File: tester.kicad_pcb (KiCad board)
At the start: 2 copper layers, 55.9 x 40.6 mm, 13 parts

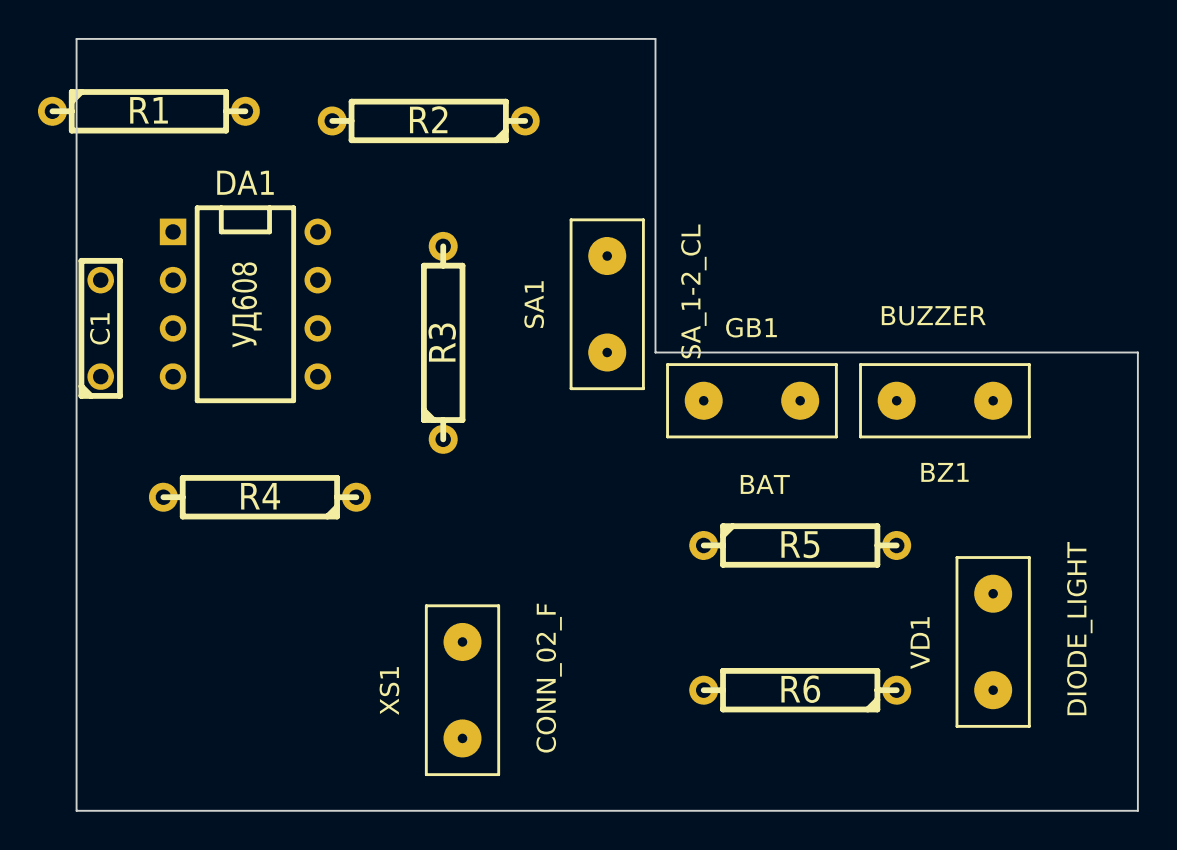
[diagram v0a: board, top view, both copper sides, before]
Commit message: next step
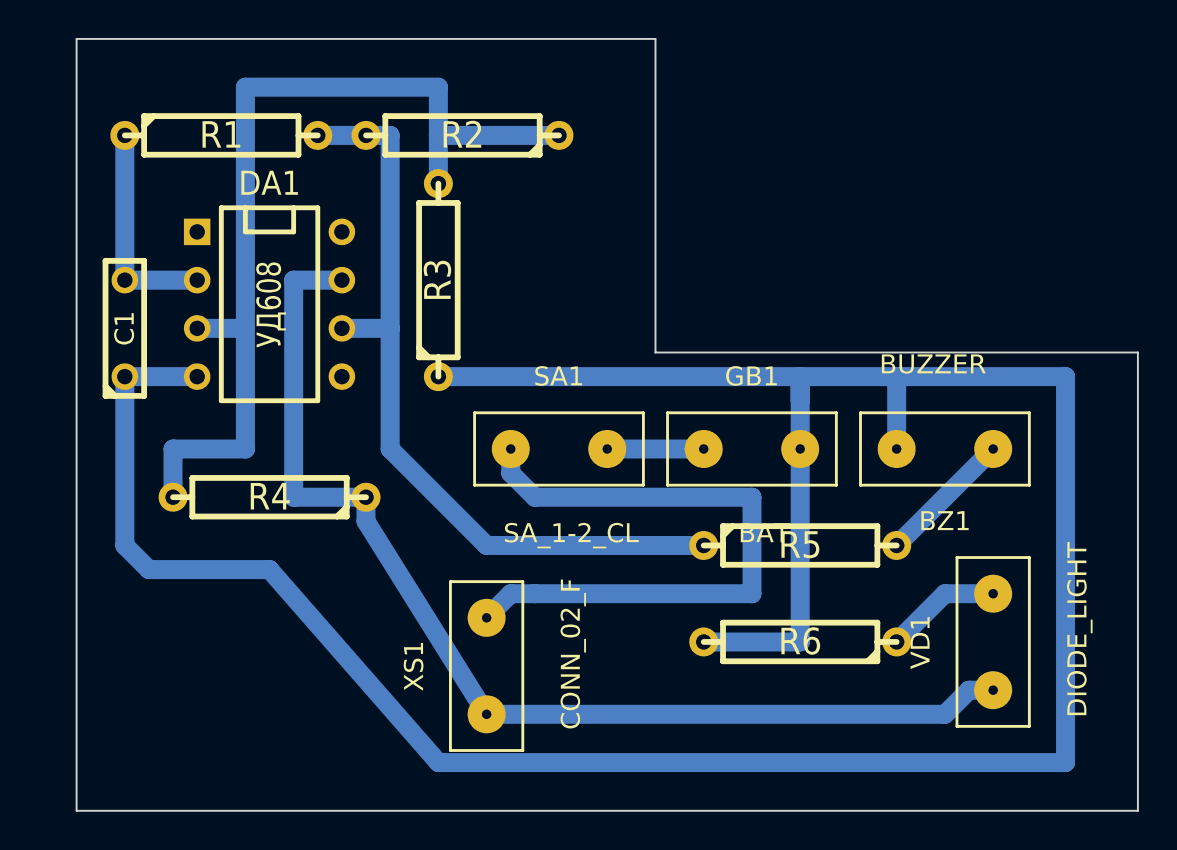
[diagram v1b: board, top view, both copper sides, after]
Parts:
- moved SA1 8.03 mm to (45.7, 55.9), turned to 0 degrees
- moved R1 4.02 mm to (27.9, 39.4)
- moved R3 3.31 mm to (39.4, 47.0)
- moved BZ1 2.54 mm to (66.0, 55.9)
- moved GB1 2.54 mm to (55.9, 55.9)
- moved R6 2.54 mm to (58.4, 66.0)
- moved R2 1.93 mm to (40.6, 39.4)
- moved XS1 1.80 mm to (41.9, 67.3)
- moved C1 1.27 mm to (22.9, 49.5)
- moved DA1 1.27 mm to (30.5, 48.3)
- moved R4 0.51 mm to (30.5, 58.4)
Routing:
- net GND: track 0.00 -> 144.8 mm
- net N-000008: track 0.00 -> 58.2 mm
- net N-000004: track 0.00 -> 49.5 mm
- net N-000009: track 0.00 -> 41.5 mm
- net N-000001: track 0.00 -> 34.1 mm
- net N-000007: track 0.00 -> 11.4 mm
- net N-000005: track 0.00 -> 7.18 mm
- net N-000002: track 0.00 -> 6.13 mm
- net N-000003: track 0.00 -> 5.08 mm
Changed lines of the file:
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@@
-(kicad_pcb (version 3) (host pcbnew "(2013-jul-07)-stable")
+(kicad_pcb (version 3) (host pcbnew "(2013-07-07 BZR 4022)-stable")
   (general
     (links 20)
-    (no_connects 20)
-    (area 20.269999 34.137599 78.486 78.934)
+    (no_connects 0)
+    (area 18.034 34.239999 76.250001 74.980001)
     (thickness 1.6)
     (drawings 6)
-    (tracks 0)
+    (tracks 53)
     (zones 0)
     (modules 13)
@@
   )
   (setup
-    (last_trace_width 0.254)
+    (last_trace_width 1)
+    (user_trace_width 0.5)
+    (user_trace_width 1)
     (trace_clearance 0.254)
     (zone_clearance 0.508)
@@
     (pad_to_mask_clearance 0)
     (aux_axis_origin 0 0)
-    (visible_elements 7FFFF591)
+    (visible_elements 7FFF2511)
     (pcbplotparams
       (layerselection 3178497)
@@
   )
   (module R4   placed (layer F.Cu)
-    (at 24.13 38.1)
+    (at 27.94 39.37)
     (descr "Resitance 4 pas")
     (tags R)
@@
   )
   (module R4   placed (layer F.Cu)
-    (at 39.624 50.292 90)
+    (at 39.37 46.99 90)
     (descr "Resitance 4 pas")
     (tags R)
@@
   )
   (module R4   placed (layer F.Cu)
-    (at 29.972 58.42 180)
+    (at 30.48 58.42 180)
     (descr "Resitance 4 pas")
     (tags R)
@@
   )
   (module R4   placed (layer F.Cu)
-    (at 38.862 38.608 180)
+    (at 40.64 39.37 180)
     (descr "Resitance 4 pas")
     (tags R)
@@
   )
   (module DIP-8__300   placed (layer F.Cu)
-    (at 29.21 48.26 270)
+    (at 30.48 48.26 270)
     (descr "8 pins DIL package, round pads")
     (tags DIL)
@@
   )
   (module C2   placed (layer F.Cu)
-    (at 21.59 49.53 90)
+    (at 22.86 49.53 90)
     (descr "Condensateur = 2 pas")
     (tags C)
@@
   )
   (module R4 (layer F.Cu)
-    (at 58.42 68.58 180)
+    (at 58.42 66.04 180)
     (descr "Resitance 4 pas")
     (tags R)
@@
   )
   (module Con2 (layer F.Cu)
-    (at 55.88 53.34)
+    (at 55.88 55.88)
     (fp_text reference GB1 (at 0 -3.81) (layer F.SilkS)
       (effects (font (size 1 1) (thickness 0.15)))
@@
   )
   (module Con2 (layer F.Cu)
-    (at 40.64 68.58 90)
+    (at 41.91 67.31 90)
     (fp_text reference XS1 (at 0 -3.81 90) (layer F.SilkS)
       (effects (font (size 1 1) (thickness 0.15)))
@@
   )
   (module Con2 (layer F.Cu)
-    (at 48.26 48.26 90)
-    (fp_text reference SA1 (at 0 -3.81 90) (layer F.SilkS)
-      (effects (font (size 1 1) (thickness 0.15)))
-    )
-    (fp_text value SA_1-2_CL (at 0.635 4.445 90) (layer F.SilkS)
+    (at 45.72 55.88)
+    (fp_text reference SA1 (at 0 -3.81) (layer F.SilkS)
+      (effects (font (size 1 1) (thickness 0.15)))
+    )
+    (fp_text value SA_1-2_CL (at 0.635 4.445) (layer F.SilkS)
+      (effects (font (size 1 1) (thickness 0.15)))
+    )
+    (fp_line (start -4.445 -1.905) (end 4.445 -1.905) (layer F.SilkS) (width 0.15))
+    (fp_line (start 4.445 -1.905) (end 4.445 1.905) (layer F.SilkS) (width 0.15))
+    (fp_line (start 4.445 1.905) (end -4.445 1.905) (layer F.SilkS) (width 0.15))
+    (fp_line (start -4.445 1.905) (end -4.445 -1.905) (layer F.SilkS) (width 0.15))
+    (pad 1 thru_hole circle (at -2.54 0) (size 2 2) (drill 0.5)
+      (layers *.Cu *.Mask F.SilkS)
+      (net 2 N-000001)
+    )
+    (pad 2 thru_hole circle (at 2.54 0) (size 2 2) (drill 0.5)
+      (layers *.Cu *.Mask F.SilkS)
+      (net 4 N-000003)
+    )
+  )
+  (module Con2 (layer F.Cu)
+    (at 68.58 66.04 90)
+    (fp_text reference VD1 (at 0 -3.81 90) (layer F.SilkS)
+      (effects (font (size 1 1) (thickness 0.15)))
+    )
+    (fp_text value DIODE_LIGHT (at 0.635 4.445 90) (layer F.SilkS)
       (effects (font (size 1 1) (thickness 0.15)))
     )
@@
     (pad 1 thru_hole circle (at -2.54 0 90) (size 2 2) (drill 0.5)
       (layers *.Cu *.Mask F.SilkS)
-      (net 2 N-000001)
+      (net 8 N-000008)
     )
     (pad 2 thru_hole circle (at 2.54 0 90) (size 2 2) (drill 0.5)
       (layers *.Cu *.Mask F.SilkS)
-      (net 4 N-000003)
+      (net 3 N-000002)
     )
   )
   (module Con2 (layer F.Cu)
-    (at 68.58 66.04 90)
-    (fp_text reference VD1 (at 0 -3.81 90) (layer F.SilkS)
-      (effects (font (size 1 1) (thickness 0.15)))
-    )
-    (fp_text value DIODE_LIGHT (at 0.635 4.445 90) (layer F.SilkS)
-      (effects (font (size 1 1) (thickness 0.15)))
-    )
-    (fp_line (start -4.445 -1.905) (end 4.445 -1.905) (layer F.SilkS) (width 0.15))
-    (fp_line (start 4.445 -1.905) (end 4.445 1.905) (layer F.SilkS) (width 0.15))
-    (fp_line (start 4.445 1.905) (end -4.445 1.905) (layer F.SilkS) (width 0.15))
-    (fp_line (start -4.445 1.905) (end -4.445 -1.905) (layer F.SilkS) (width 0.15))
-    (pad 1 thru_hole circle (at -2.54 0 90) (size 2 2) (drill 0.5)
-      (layers *.Cu *.Mask F.SilkS)
-      (net 8 N-000008)
-    )
-    (pad 2 thru_hole circle (at 2.54 0 90) (size 2 2) (drill 0.5)
-      (layers *.Cu *.Mask F.SilkS)
-      (net 3 N-000002)
-    )
-  )
-  (module Con2 (layer F.Cu)
-    (at 66.04 53.34 180)
+    (at 66.04 55.88 180)
     (fp_text reference BZ1 (at 0 -3.81 180) (layer F.SilkS)
       (effects (font (size 1 1) (thickness 0.15)))
@@
   (gr_line (start 20.32 74.93) (end 76.2 74.93) (angle 90) (layer Edge.Cuts) (width 0.1))
   (gr_line (start 20.32 34.29) (end 20.32 74.93) (angle 90) (layer Edge.Cuts) (width 0.1))
+  (segment (start 22.86 52.07) (end 22.86 60.96) (width 1) (layer B.Cu) (net 1))
+  (segment (start 72.39 52.07) (end 63.5 52.07) (width 1) (layer B.Cu) (net 1))
+  (segment (start 72.39 72.39) (end 72.39 52.07) (width 1) (layer B.Cu) (net 1))
+  (segment (start 39.37 72.39) (end 72.39 72.39) (width 1) (layer B.Cu) (net 1))
+  (segment (start 30.48 62.23) (end 39.37 72.39) (width 1) (layer B.Cu) (net 1))
+  (segment (start 24.13 62.23) (end 30.48 62.23) (width 1) (layer B.Cu) (net 1))
+  (segment (start 22.86 60.96) (end 24.13 62.23) (width 1) (layer B.Cu) (net 1))
+  (segment (start 39.37 52.07) (end 58.42 52.07) (width 1) (layer B.Cu) (net 1))
+  (segment (start 58.42 52.07) (end 58.42 53.34) (width 1) (layer B.Cu) (net 1))
+  (segment (start 53.34 66.04) (end 58.42 66.04) (width 1) (layer B.Cu) (net 1))
+  (segment (start 58.42 66.04) (end 58.42 55.88) (width 1) (layer B.Cu) (net 1))
+  (segment (start 22.86 52.07) (end 26.67 52.07) (width 1) (layer B.Cu) (net 1))
+  (segment (start 63.5 55.88) (end 63.5 52.07) (width 1) (layer B.Cu) (net 1))
+  (segment (start 58.42 52.07) (end 58.42 53.34) (width 1) (layer B.Cu) (net 1))
+  (segment (start 58.42 53.34) (end 58.42 55.88) (width 1) (layer B.Cu) (net 1))
+  (segment (start 63.5 52.07) (end 58.42 52.07) (width 1) (layer B.Cu) (net 1))
+  (segment (start 44.45 63.5) (end 43.18 63.5) (width 1) (layer B.Cu) (net 2))
+  (segment (start 43.18 57.15) (end 44.45 58.42) (width 1) (layer B.Cu) (net 2))
+  (segment (start 44.45 58.42) (end 55.88 58.42) (width 1) (layer B.Cu) (net 2))
+  (segment (start 55.88 58.42) (end 55.88 63.5) (width 1) (layer B.Cu) (net 2))
+  (segment (start 55.88 63.5) (end 44.45 63.5) (width 1) (layer B.Cu) (net 2))
+  (segment (start 43.18 55.88) (end 43.18 57.15) (width 1) (layer B.Cu) (net 2))
+  (segment (start 43.18 63.5) (end 41.91 64.77) (width 1) (layer B.Cu) (net 2) (status 800000))
+  (segment (start 68.58 63.5) (end 66.04 63.5) (width 1) (layer B.Cu) (net 3))
+  (segment (start 66.04 63.5) (end 63.5 66.04) (width 1) (layer B.Cu) (net 3))
+  (segment (start 48.26 55.88) (end 53.34 55.88) (width 1) (layer B.Cu) (net 4))
+  (segment (start 25.4 58.42) (end 25.4 55.88) (width 1) (layer B.Cu) (net 5))
+  (segment (start 29.21 55.88) (end 29.21 49.53) (width 1) (layer B.Cu) (net 5))
+  (segment (start 25.4 55.88) (end 29.21 55.88) (width 1) (layer B.Cu) (net 5))
+  (segment (start 45.72 39.37) (end 39.37 39.37) (width 1) (layer B.Cu) (net 5))
+  (segment (start 39.37 41.91) (end 39.37 39.37) (width 1) (layer B.Cu) (net 5))
+  (segment (start 39.37 39.37) (end 39.37 36.83) (width 1) (layer B.Cu) (net 5))
+  (segment (start 29.21 49.53) (end 26.67 49.53) (width 1) (layer B.Cu) (net 5))
+  (segment (start 29.21 36.83) (end 29.21 49.53) (width 1) (layer B.Cu) (net 5))
+  (segment (start 39.37 36.83) (end 29.21 36.83) (width 1) (layer B.Cu) (net 5))
+  (segment (start 63.5 60.96) (end 68.58 55.88) (width 1) (layer B.Cu) (net 6))
+  (segment (start 22.86 46.99) (end 22.86 39.37) (width 1) (layer B.Cu) (net 7))
+  (segment (start 22.86 46.99) (end 26.67 46.99) (width 1) (layer B.Cu) (net 7))
+  (segment (start 41.91 69.85) (end 66.04 69.85) (width 1) (layer B.Cu) (net 8) (status 400000))
+  (segment (start 67.31 68.58) (end 68.58 68.58) (width 1) (layer B.Cu) (net 8) (status 800000))
+  (segment (start 66.04 69.85) (end 67.31 68.58) (width 1) (layer B.Cu) (net 8))
+  (segment (start 41.91 69.85) (end 35.56 59.69) (width 1) (layer B.Cu) (net 8) (status 400000))
+  (segment (start 35.56 59.69) (end 35.56 58.42) (width 1) (layer B.Cu) (net 8))
+  (segment (start 35.56 58.42) (end 31.75 58.42) (width 1) (layer B.Cu) (net 8))
+  (segment (start 31.75 58.42) (end 31.75 46.99) (width 1) (layer B.Cu) (net 8))
+  (segment (start 31.75 46.99) (end 34.29 46.99) (width 1) (layer B.Cu) (net 8))
+  (segment (start 36.83 49.53) (end 36.83 55.88) (width 1) (layer B.Cu) (net 9))
+  (segment (start 41.91 60.96) (end 53.34 60.96) (width 1) (layer B.Cu) (net 9))
+  (segment (start 36.83 55.88) (end 41.91 60.96) (width 1) (layer B.Cu) (net 9))
+  (segment (start 34.29 49.53) (end 36.83 49.53) (width 1) (layer B.Cu) (net 9))
+  (segment (start 36.83 39.37) (end 35.56 39.37) (width 1) (layer B.Cu) (net 9))
+  (segment (start 36.83 49.53) (end 36.83 39.37) (width 1) (layer B.Cu) (net 9))
+  (segment (start 35.56 39.37) (end 33.02 39.37) (width 1) (layer B.Cu) (net 9))
 )
